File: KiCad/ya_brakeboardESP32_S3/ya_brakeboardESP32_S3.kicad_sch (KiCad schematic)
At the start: 10 parts, among them J1 Screw_Terminal_01x04, J2 SR_0_Terminal, J3 SR_1_Terminal, J4 SR_2_Terminal, U1 TPIC6B595N, U2 TPIC6B595N, U3 TPIC6B595N

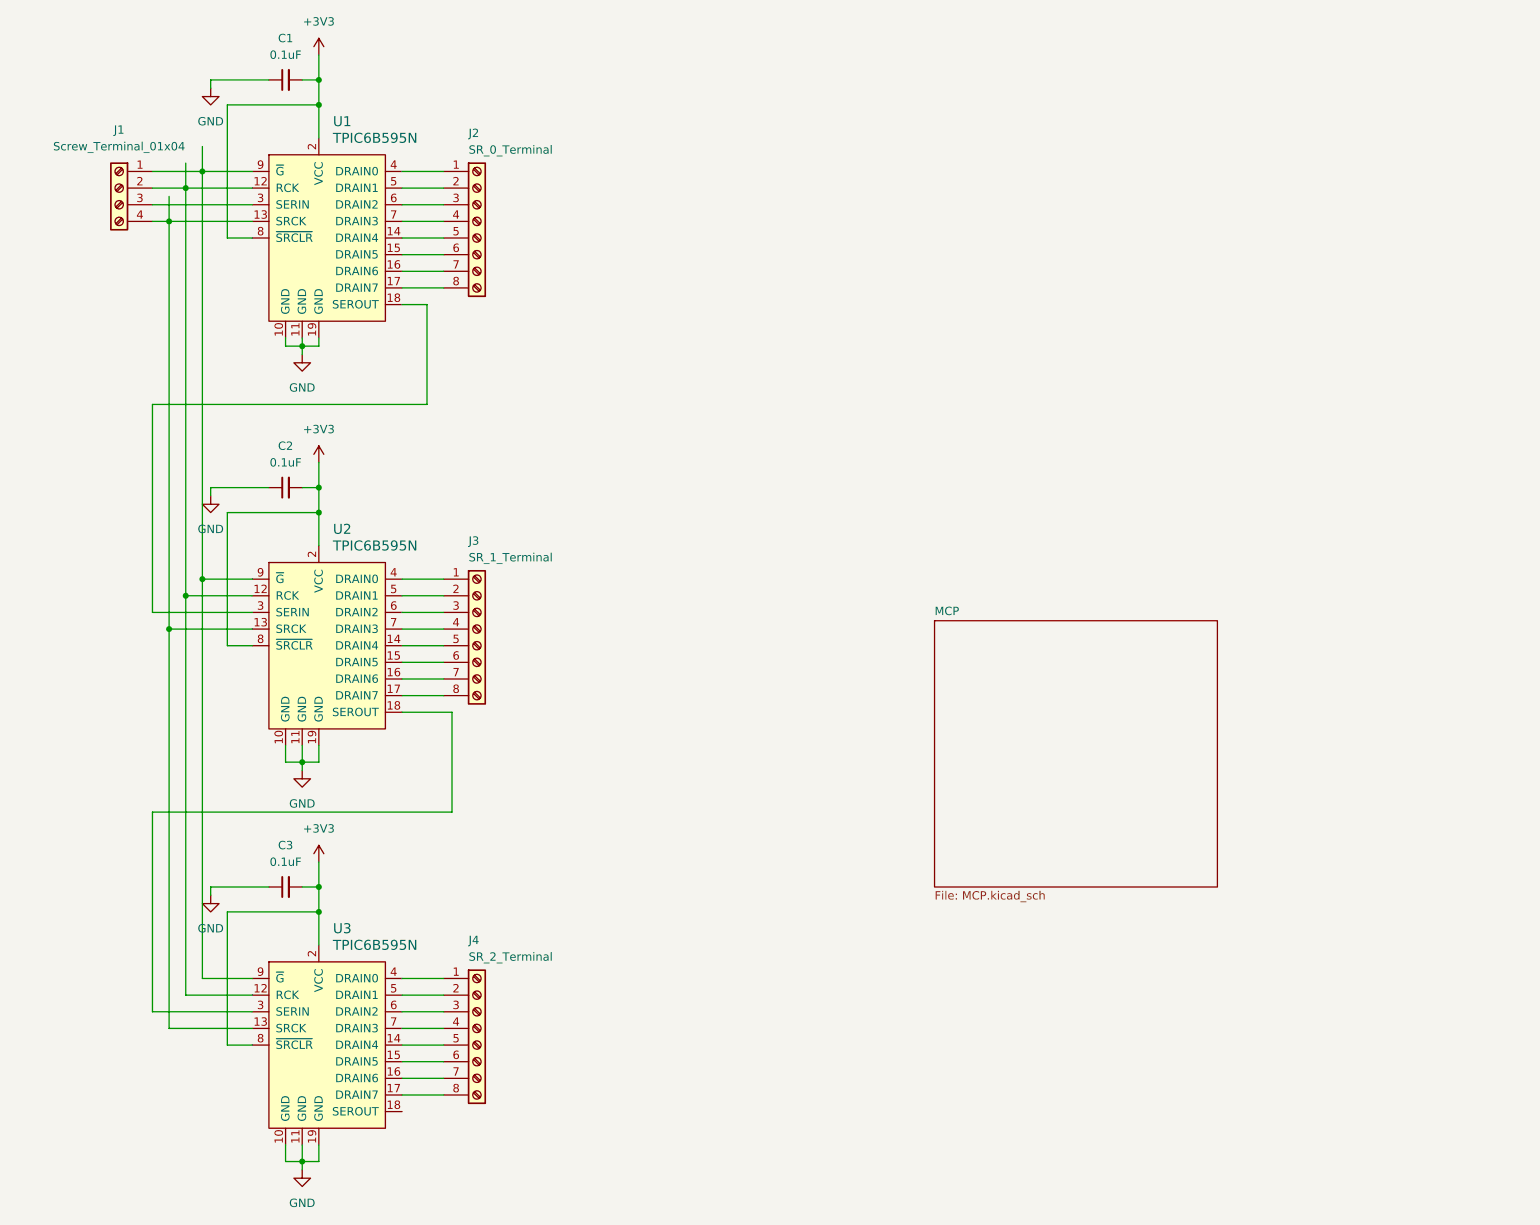
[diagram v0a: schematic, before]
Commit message: basic schematics finished
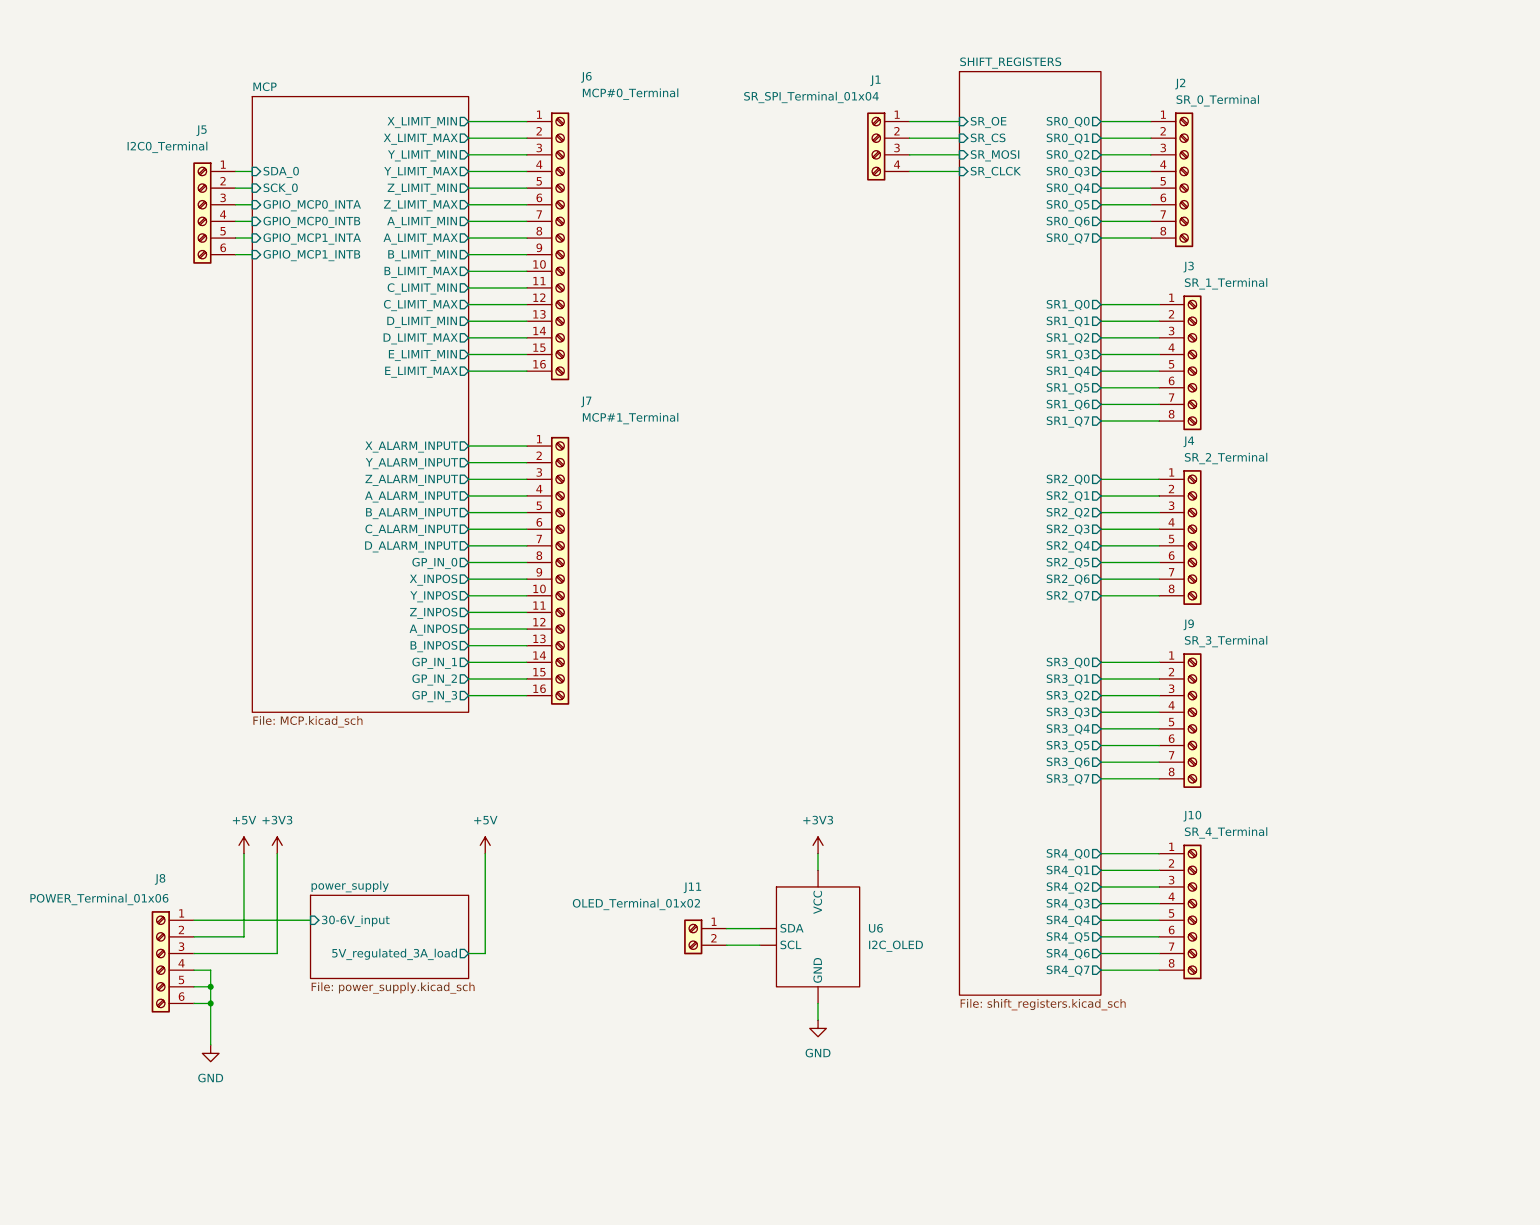
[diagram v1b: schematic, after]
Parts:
- removed C1, C2, C3: 0.1uF, symbol Device:C_Small
- removed U1, U2, U3: TPIC6B595N, digikey-footprints:DIP-20_W7.62mm, symbol dk_Logic-Shift-Registers:TPIC6B595N
- added J10: SR_4_Terminal, symbol Connector:Screw_Terminal_01x08
- added J11: OLED_Terminal_01x02, symbol Connector:Screw_Terminal_01x02
- added J5: I2C0_Terminal, symbol Connector:Screw_Terminal_01x06
- added J6: MCP#0_Terminal, symbol Connector:Screw_Terminal_01x16
- added J7: MCP#1_Terminal, symbol Connector:Screw_Terminal_01x16
- added J8: POWER_Terminal_01x06, symbol Connector:Screw_Terminal_01x06
- added J9: SR_3_Terminal, symbol Connector:Screw_Terminal_01x08
- added U6: I2C_OLED, symbol PositionerLib:I2C_Device_3V3
- J1: value Screw_Terminal_01x04 -> SR_SPI_Terminal_01x04
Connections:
- net +3V3: now also J8.3 (Pin_3), U6.3 (VCC)
- net GND: now also J8.4 (Pin_4), J8.5 (Pin_5), J8.6 (Pin_6), U6. (GND)
- net SHIFT_REGISTERS/SR1_Q0: now reaches J3.1 (Pin_1)
- net SHIFT_REGISTERS/SR1_Q1: now reaches J3.2 (Pin_2)
- net SHIFT_REGISTERS/SR1_Q2: now reaches J3.3 (Pin_3)
- net SHIFT_REGISTERS/SR1_Q3: now reaches J3.4 (Pin_4)
- net SHIFT_REGISTERS/SR1_Q4: now reaches J3.5 (Pin_5)
- net SHIFT_REGISTERS/SR1_Q5: now reaches J3.6 (Pin_6)
- net SHIFT_REGISTERS/SR1_Q6: now reaches J3.7 (Pin_7)
- net SHIFT_REGISTERS/SR1_Q7: now reaches J3.8 (Pin_8)
- net SHIFT_REGISTERS/SR_OE: now reaches J1.1 (Pin_1)
- net SHIFT_REGISTERS/SR_CS: now reaches J1.2 (Pin_2)
- net SHIFT_REGISTERS/SR_MOSI: now reaches J1.3 (Pin_3)
- net SHIFT_REGISTERS/SR_CLCK: now reaches J1.4 (Pin_4)
- net SHIFT_REGISTERS/SR2_Q4: now reaches J4.5 (Pin_5)
- net SHIFT_REGISTERS/SR2_Q5: now reaches J4.6 (Pin_6)
- net SHIFT_REGISTERS/SR2_Q6: now reaches J4.7 (Pin_7)
- net SHIFT_REGISTERS/SR2_Q7: now reaches J4.8 (Pin_8)
- net SHIFT_REGISTERS/SR2_Q0: now reaches J4.1 (Pin_1)
- net SHIFT_REGISTERS/SR2_Q1: now reaches J4.2 (Pin_2)
- net SHIFT_REGISTERS/SR2_Q2: now reaches J4.3 (Pin_3)
- net SHIFT_REGISTERS/SR2_Q3: now reaches J4.4 (Pin_4)
- net SHIFT_REGISTERS/SR0_Q0: now reaches J2.1 (Pin_1)
- net SHIFT_REGISTERS/SR0_Q1: now reaches J2.2 (Pin_2)
- net SHIFT_REGISTERS/SR0_Q2: now reaches J2.3 (Pin_3)
- net SHIFT_REGISTERS/SR0_Q3: now reaches J2.4 (Pin_4)
- net SHIFT_REGISTERS/SR0_Q4: now reaches J2.5 (Pin_5)
- net SHIFT_REGISTERS/SR0_Q5: now reaches J2.6 (Pin_6)
- net SHIFT_REGISTERS/SR0_Q6: now reaches J2.7 (Pin_7)
- net SHIFT_REGISTERS/SR0_Q7: now reaches J2.8 (Pin_8)
- new net: J11.1 (Pin_1), U6.1 (SDA)
- new net: J11.2 (Pin_2), U6.2 (SCL)
- new net +5V: J8.2 (Pin_2)
- new net MCP/A_ALARM_INPUT: J7.4 (Pin_4)
- new net MCP/A_INPOS: J7.12 (Pin_12)
- new net MCP/A_LIMIT_MAX: J6.8 (Pin_8)
- new net MCP/A_LIMIT_MIN: J6.7 (Pin_7)
- new net MCP/B_ALARM_INPUT: J7.5 (Pin_5)
- new net MCP/B_INPOS: J7.13 (Pin_13)
- new net MCP/B_LIMIT_MAX: J6.10 (Pin_10)
- new net MCP/B_LIMIT_MIN: J6.9 (Pin_9)
- new net MCP/C_ALARM_INPUT: J7.6 (Pin_6)
- new net MCP/C_LIMIT_MAX: J6.12 (Pin_12)
- new net MCP/C_LIMIT_MIN: J6.11 (Pin_11)
- new net MCP/D_ALARM_INPUT: J7.7 (Pin_7)
- new net MCP/D_LIMIT_MAX: J6.14 (Pin_14)
- new net MCP/D_LIMIT_MIN: J6.13 (Pin_13)
- new net MCP/E_LIMIT_MAX: J6.16 (Pin_16)
- new net MCP/E_LIMIT_MIN: J6.15 (Pin_15)
- new net MCP/GPIO_MCP0_INTA: J5.3 (Pin_3)
- new net MCP/GPIO_MCP0_INTB: J5.4 (Pin_4)
- new net MCP/GPIO_MCP1_INTA: J5.5 (Pin_5)
- new net MCP/GPIO_MCP1_INTB: J5.6 (Pin_6)
- new net MCP/GP_IN_0: J7.8 (Pin_8)
- new net MCP/GP_IN_1: J7.14 (Pin_14)
- new net MCP/GP_IN_2: J7.15 (Pin_15)
- new net MCP/GP_IN_3: J7.16 (Pin_16)
- new net MCP/SCK_0: J5.2 (Pin_2)
- new net MCP/SDA_0: J5.1 (Pin_1)
- new net MCP/X_ALARM_INPUT: J7.1 (Pin_1)
- new net MCP/X_INPOS: J7.9 (Pin_9)
- new net MCP/X_LIMIT_MAX: J6.2 (Pin_2)
- new net MCP/X_LIMIT_MIN: J6.1 (Pin_1)
- new net MCP/Y_ALARM_INPUT: J7.2 (Pin_2)
- new net MCP/Y_INPOS: J7.10 (Pin_10)
- new net MCP/Y_LIMIT_MAX: J6.4 (Pin_4)
- new net MCP/Y_LIMIT_MIN: J6.3 (Pin_3)
- new net MCP/Z_ALARM_INPUT: J7.3 (Pin_3)
- new net MCP/Z_INPOS: J7.11 (Pin_11)
- new net MCP/Z_LIMIT_MAX: J6.6 (Pin_6)
- new net MCP/Z_LIMIT_MIN: J6.5 (Pin_5)
- new net SHIFT_REGISTERS/SR3_Q0: J9.1 (Pin_1)
- new net SHIFT_REGISTERS/SR3_Q1: J9.2 (Pin_2)
- new net SHIFT_REGISTERS/SR3_Q2: J9.3 (Pin_3)
- new net SHIFT_REGISTERS/SR3_Q3: J9.4 (Pin_4)
- new net SHIFT_REGISTERS/SR3_Q4: J9.5 (Pin_5)
- new net SHIFT_REGISTERS/SR3_Q5: J9.6 (Pin_6)
- new net SHIFT_REGISTERS/SR3_Q6: J9.7 (Pin_7)
- new net SHIFT_REGISTERS/SR3_Q7: J9.8 (Pin_8)
- new net SHIFT_REGISTERS/SR4_Q0: J10.1 (Pin_1)
- new net SHIFT_REGISTERS/SR4_Q1: J10.2 (Pin_2)
- new net SHIFT_REGISTERS/SR4_Q2: J10.3 (Pin_3)
- new net SHIFT_REGISTERS/SR4_Q3: J10.4 (Pin_4)
- new net SHIFT_REGISTERS/SR4_Q4: J10.5 (Pin_5)
- new net SHIFT_REGISTERS/SR4_Q5: J10.6 (Pin_6)
- new net SHIFT_REGISTERS/SR4_Q6: J10.7 (Pin_7)
- new net SHIFT_REGISTERS/SR4_Q7: J10.8 (Pin_8)
- new net power_supply/30-6V_input: J8.1 (Pin_1)
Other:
- added sheet SHIFT_REGISTERS (shift_registers.kicad_sch)
- added sheet power_supply (power_supply.kicad_sch)
- sheet MCP ports: added A_ALARM_INPUT, A_INPOS, A_LIMIT_MAX, A_LIMIT_MIN, B_ALARM_INPUT, B_INPOS, B_LIMIT_MAX, B_LIMIT_MIN, C_ALARM_INPUT, C_LIMIT_MAX, C_LIMIT_MIN, D_ALARM_INPUT, D_LIMIT_MAX, D_LIMIT_MIN, E_LIMIT_MAX, E_LIMIT_MIN, GPIO_MCP0_INTA, GPIO_MCP0_INTB, GPIO_MCP1_INTA, GPIO_MCP1_INTB, GP_IN_0, GP_IN_1, GP_IN_2, GP_IN_3, SCK_0, SDA_0, X_ALARM_INPUT, X_INPOS, X_LIMIT_MAX, X_LIMIT_MIN, Y_ALARM_INPUT, Y_INPOS, Y_LIMIT_MAX, Y_LIMIT_MIN, Z_ALARM_INPUT, Z_INPOS, Z_LIMIT_MAX, Z_LIMIT_MIN; removed none
- moved on the sheet: J1, J2, J3, J4

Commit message: ready for implementation
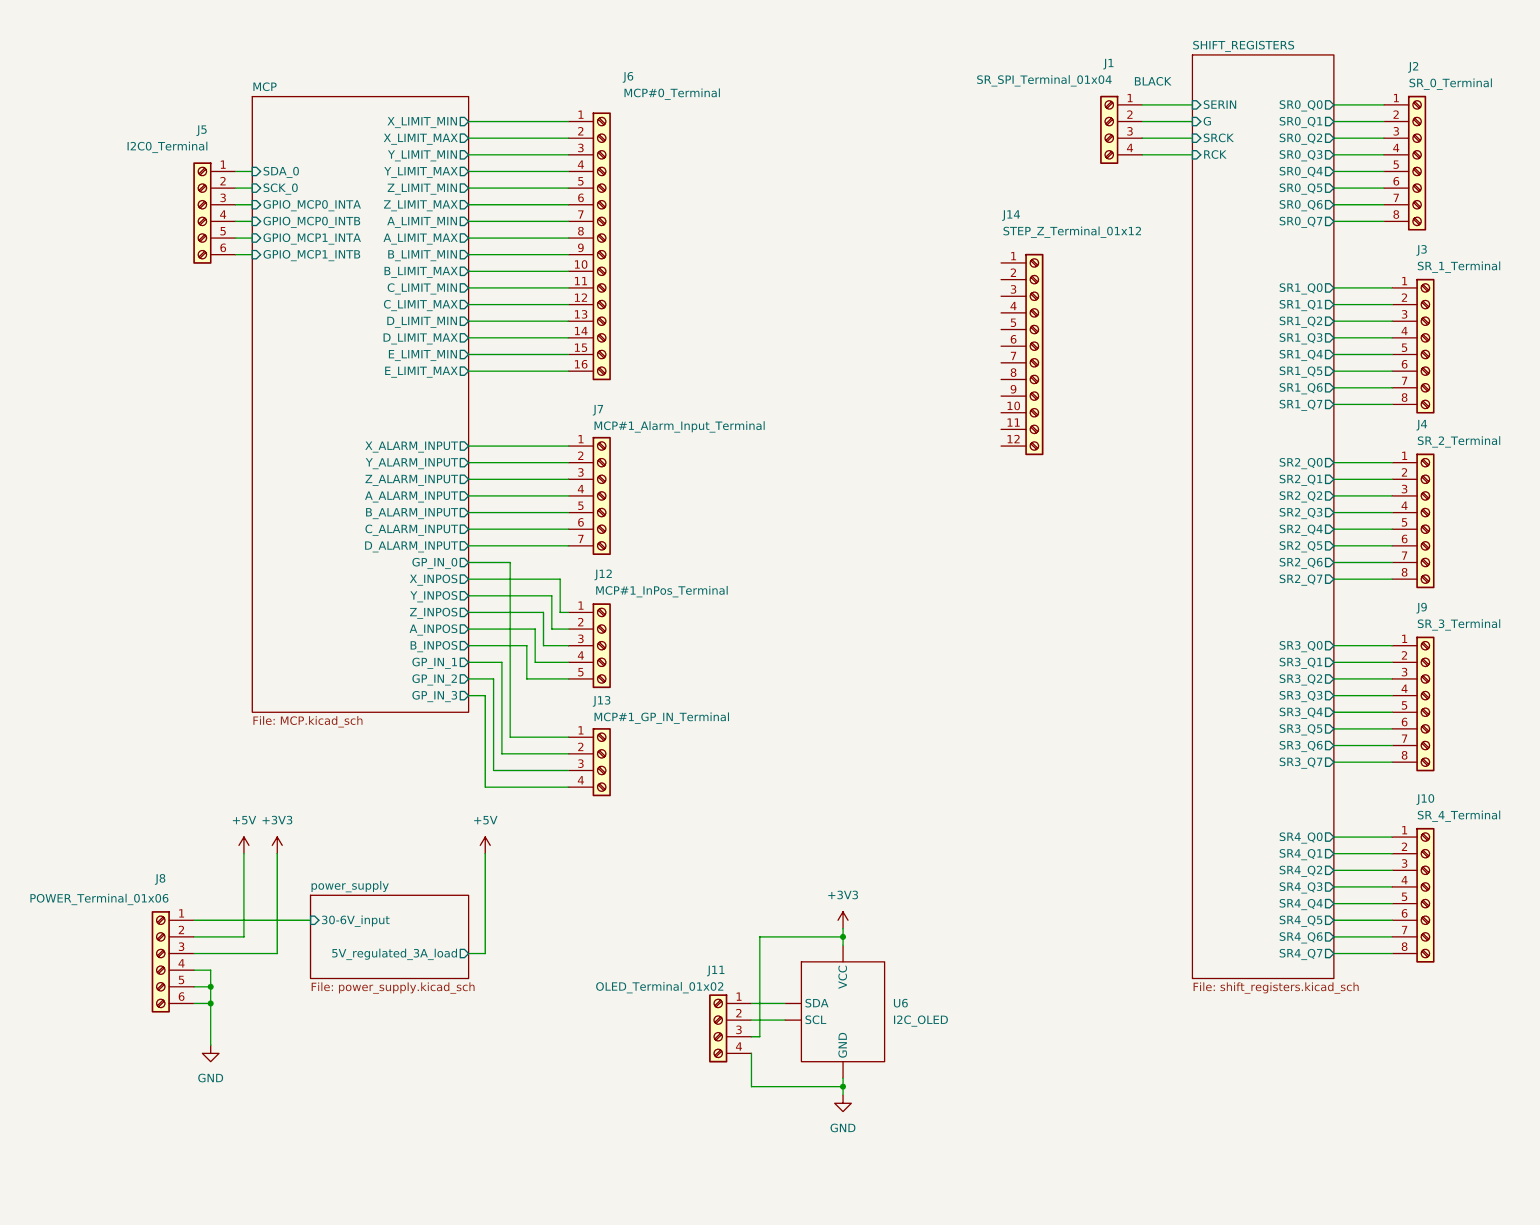
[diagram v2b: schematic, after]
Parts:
- added J12: MCP#1_InPos_Terminal, symbol Connector:Screw_Terminal_01x05
- added J13: MCP#1_GP_IN_Terminal, symbol Connector:Screw_Terminal_01x04
- added J14: STEP_Z_Terminal_01x12, symbol Connector:Screw_Terminal_01x12
- J11: symbol Connector:Screw_Terminal_01x02 -> Connector:Screw_Terminal_01x04
- J7: value MCP#1_Terminal -> MCP#1_Alarm_Input_Terminal; symbol Connector:Screw_Terminal_01x16 -> Connector:Screw_Terminal_01x07
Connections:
- net +3V3: now also J11.3 (Pin_3)
- net GND: now also J11.4 (Pin_4)
- net MCP/A_INPOS: now also J12.4 (Pin_4); no longer J7.12 (Pin_12)
- net MCP/B_INPOS: now also J12.5 (Pin_5); no longer J7.13 (Pin_13)
- net MCP/GP_IN_0: now also J13.1 (Pin_1); no longer J7.8 (Pin_8)
- net MCP/GP_IN_1: now also J13.2 (Pin_2); no longer J7.14 (Pin_14)
- net MCP/GP_IN_2: now also J13.3 (Pin_3); no longer J7.15 (Pin_15)
- net MCP/GP_IN_3: now also J13.4 (Pin_4); no longer J7.16 (Pin_16)
- net MCP/X_INPOS: now also J12.1 (Pin_1); no longer J7.9 (Pin_9)
- net MCP/Y_INPOS: now also J12.2 (Pin_2); no longer J7.10 (Pin_10)
- net MCP/Z_INPOS: now also J12.3 (Pin_3); no longer J7.11 (Pin_11)
- net SHIFT_REGISTERS/SR_CLCK renamed SHIFT_REGISTERS/RCK
- net SHIFT_REGISTERS/SR_CS renamed SHIFT_REGISTERS/G
- net SHIFT_REGISTERS/SR_MOSI renamed SHIFT_REGISTERS/SRCK
- net SHIFT_REGISTERS/SR_OE renamed SHIFT_REGISTERS/SERIN
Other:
- sheet SHIFT_REGISTERS ports: added G, RCK, SERIN, SRCK; removed SR_CLCK, SR_CS, SR_MOSI, SR_OE
- note added: "BLACK"
- moved on the sheet: J1, J10, J2, J3, J4, J6, J9, U6
